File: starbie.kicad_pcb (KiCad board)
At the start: 2 copper layers, 125 x 100.5 mm, 9 parts, among them J1 Conn_01x04_Pin, J2 Conn_01x08_Pin, SW1 SW_Push, SW2 SW_Push, U1 XIAO-ESP32-C3-SMD, U2 DHT11

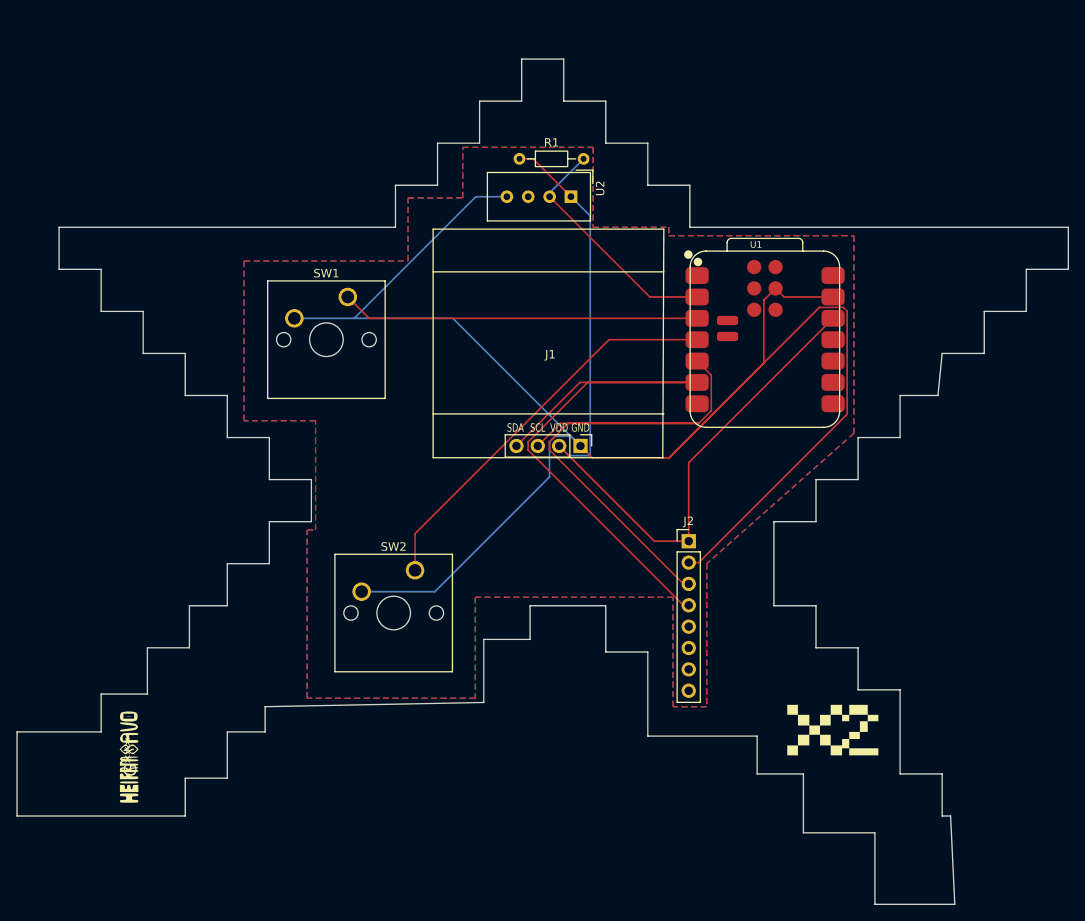
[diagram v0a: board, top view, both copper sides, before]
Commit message: fix PCB design
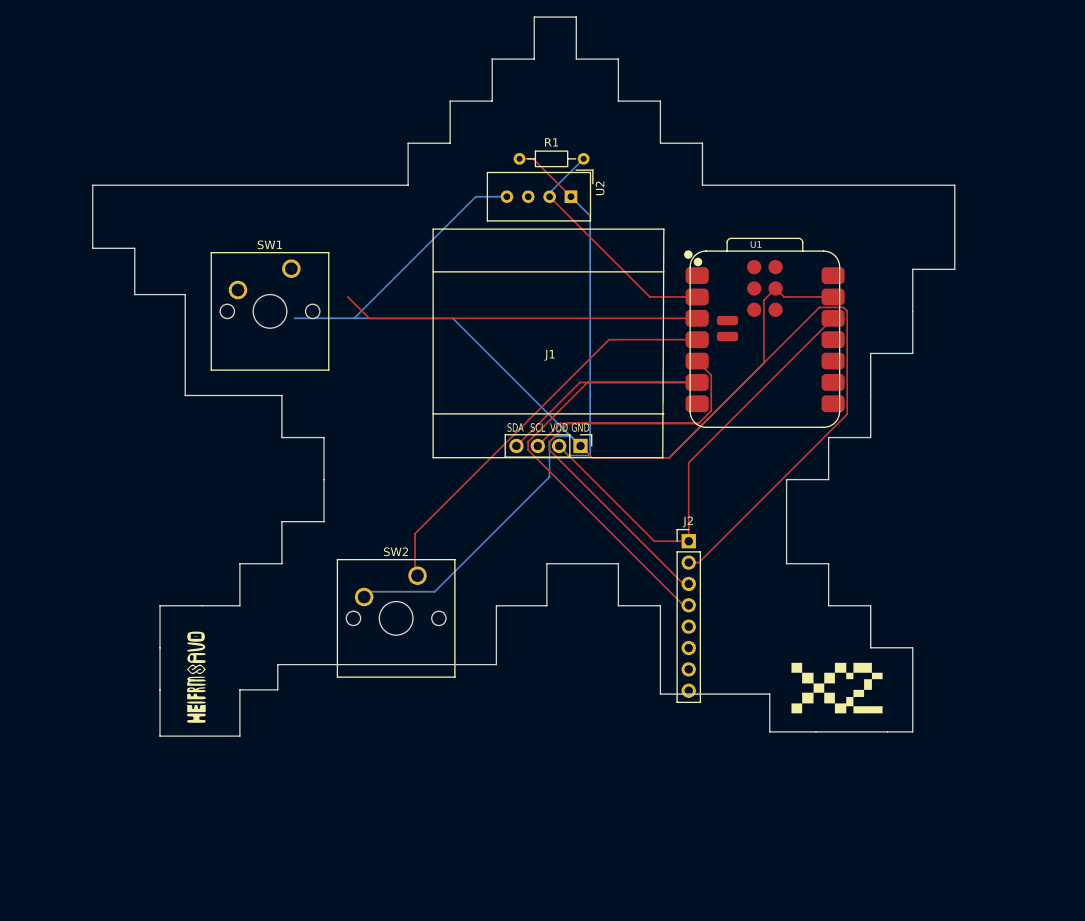
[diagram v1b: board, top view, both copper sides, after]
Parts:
- moved G*** 12.4 mm to (81.5, 133.5)
- moved SW1 7.50 mm to (92.6, 84.9)
- moved G*** 5.02 mm to (157.5, 135.0)
- moved SW2 0.70 mm to (107.6, 121.4)
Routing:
- removed copper zone on B.Cu, net GND
- removed copper zone on F.Cu, net GND
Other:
- board size 125 x 100.5 mm -> 102.5 x 85.5 mm
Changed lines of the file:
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@@
 	(footprint "graphics:x2logo"
 		(layer "F.Cu")
-		(at 157 140)
+		(at 157.5 135)
 		(property "Reference" "G***"
 			(at 0 0 0)
@@
 	(footprint "graphics:hello"
 		(layer "F.Cu")
-		(at 73.5 143 90)
+		(at 81.5 133.5 90)
 		(property "Reference" "G***"
 			(at 0 0 90)
 			(layer "F.SilkS")
+			(hide yes)
 			(effects
 				(font
@@
 	(footprint "Button_Switch_Keyboard:SW_Cherry_MX_1.00u_PCB"
 		(layer "F.Cu")
-		(at 107.326 120.785)
+		(at 107.62 121.42)
 		(descr "Cherry MX keyswitch, 1.00u, PCB mount, http://cherryamericas.com/wp-content/uploads/2014/12/mx_cat.pdf")
 		(tags "Cherry MX keyswitch 1.00u PCB")
@@
 	(footprint "Button_Switch_Keyboard:SW_Cherry_MX_1.00u_PCB"
 		(layer "F.Cu")
-		(at 99.326 88.285)
+		(at 92.62 84.92)
 		(descr "Cherry MX keyswitch, 1.00u, PCB mount, http://cherryamericas.com/wp-content/uploads/2014/12/mx_cat.pdf")
 		(tags "Cherry MX keyswitch 1.00u PCB")
@@
 	(gr_poly
 		(pts
-			(xy 130 125) (xy 130 130.5) (xy 135 130.5) (xy 135 140.5) (xy 148 140.5) (xy 148 145) (xy 153.5 145)
-			(xy 153.5 152) (xy 162 152) (xy 162 160.5) (xy 171.5 160.5) (xy 171 150) (xy 170 150) (xy 170 145)
-			(xy 165 145) (xy 165 135) (xy 160 135) (xy 160 130) (xy 155 130) (xy 155 125) (xy 150 125) (xy 150 115)
-			(xy 155 115) (xy 155 110) (xy 160 110) (xy 160 105) (xy 165 105) (xy 165 100) (xy 169.5 100) (xy 170 95)
-			(xy 175 95) (xy 175 90) (xy 180 90) (xy 180 85) (xy 185 85) (xy 185 80) (xy 140 80) (xy 140 75) (xy 135 75)
-			(xy 135 70) (xy 130 70) (xy 130 65) (xy 125 65) (xy 125 60) (xy 120 60) (xy 120 65) (xy 115 65) (xy 115 70)
-			(xy 110 70) (xy 110 75) (xy 105 75) (xy 105 80) (xy 65 80) (xy 65 85) (xy 70 85) (xy 70 90) (xy 75 90)
-			(xy 75 95) (xy 80 95) (xy 80 100) (xy 85 100) (xy 85 105) (xy 90 105) (xy 90 110) (xy 95 110) (xy 95 115)
-			(xy 90 115) (xy 90 120) (xy 85 120) (xy 85 125) (xy 80.5 125) (xy 80.5 130) (xy 75.5 130) (xy 75.5 135.5)
-			(xy 70 135.5) (xy 70 140) (xy 60 140) (xy 60 150) (xy 80 150) (xy 80 145.5) (xy 85 145.5) (xy 85 140)
-			(xy 89.5 140) (xy 89.5 137) (xy 115.5 136.5) (xy 115.5 129) (xy 121 129) (xy 121 125)
+			(xy 131.5 120) (xy 131.5 125) (xy 136.5 125) (xy 136.5 135.5) (xy 149.5 135.5) (xy 149.5 140) (xy 155 140)
+			(xy 163.5 140) (xy 166.5 140) (xy 166.5 130) (xy 161.5 130) (xy 161.5 125) (xy 156.5 125) (xy 156.5 120)
+			(xy 151.5 120) (xy 151.5 110) (xy 156.5 110) (xy 156.5 105) (xy 161.5 105) (xy 161.5 100) (xy 161.5 95)
+			(xy 166.5 95) (xy 166.5 90) (xy 166.5 85) (xy 171.5 85) (xy 171.5 75) (xy 141.5 75) (xy 141.5 70)
+			(xy 136.5 70) (xy 136.5 65) (xy 131.5 65) (xy 131.5 60) (xy 126.5 60) (xy 126.5 55) (xy 121.5 55)
+			(xy 121.5 60) (xy 116.5 60) (xy 116.5 65) (xy 111.5 65) (xy 111.5 70) (xy 106.5 70) (xy 106.5 75)
+			(xy 69 75) (xy 69 82.5) (xy 74 82.5) (xy 74 88) (xy 80 88) (xy 80 100) (xy 91.5 100) (xy 91.5 105)
+			(xy 96.5 105) (xy 96.5 110) (xy 96.5 115) (xy 91.5 115) (xy 91.5 120) (xy 86.5 120) (xy 86.5 125)
+			(xy 82 125) (xy 77 125) (xy 77 130) (xy 77 135) (xy 77 140.5) (xy 86.5 140.5) (xy 86.5 135) (xy 91 135)
+			(xy 91 132) (xy 117 132) (xy 117 125) (xy 123 125) (xy 123 120)
 		)
 		(stroke
@@
 	)
 	(gr_text "Original design by SharKingStudios\nBrought to you by yours truly, Ada (asmx2)"
-		(at 184 84 0)
+		(at 170.5 79 0)
 		(layer "B.SilkS")
 		(effects
@@
 		(net "/GPIO3")
 	)
-	(zone
-		(net "GND")
-		(layers "F.Cu" "B.Cu")
-		(hatch edge 0.5)
-		(connect_pads
-			(clearance 0.5)
-		)
-		(min_thickness 0.25)
-		(fill
-			(thermal_gap 0.5)
-			(thermal_bridge_width 0.5)
-			(island_removal_mode 0)
-		)
-		(polygon
-			(pts
-				(xy 106.5 84) (xy 106.5 76.5) (xy 113 76.5) (xy 113 70.5) (xy 128.5 70.5) (xy 128.5 80) (xy 137.5 80)
-				(xy 137.5 81) (xy 159.5 81) (xy 159.5 104.5) (xy 142 120) (xy 142 137) (xy 138 137) (xy 138 124)
-				(xy 114.5 124) (xy 114.5 136) (xy 94.5 136) (xy 94.5 116) (xy 95.5 116) (xy 95.5 103) (xy 87 103)
-				(xy 87 84)
-			)
-		)
-	)
 	(embedded_fonts no)
